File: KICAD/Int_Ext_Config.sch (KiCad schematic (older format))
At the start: 7 parts

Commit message: a ton of new stuff. V0.8
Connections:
- net labels added: +6V, +7V
- net labels removed: +2V5, VCC
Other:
- note added: "A voir au dernier moment"
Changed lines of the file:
@@
 $Descr A4 11693 8268
 encoding utf-8
-Sheet 8 15
+Sheet 8 16
 Title ""
 Date ""
@@
 Wire Wire Line
 	5450 3950 5450 4050
-$Comp
-L power:VCC #PWR0110
-U 1 1 618860AB
-P 5450 3950
-F 0 "#PWR0110" H 5450 3800 50  0001 C CNN
-F 1 "VCC" H 5465 4123 50  0000 C CNN
-F 2 "" H 5450 3950 50  0001 C CNN
-F 3 "" H 5450 3950 50  0001 C CNN
-	1    5450 3950
-	1    0    0    -1
-$EndComp
-$Comp
-L power:+2V5 #PWR0111
-U 1 1 618860B1
-P 5650 3950
-F 0 "#PWR0111" H 5650 3800 50  0001 C CNN
-F 1 "+2V5" H 5665 4123 50  0000 C CNN
-F 2 "" H 5650 3950 50  0001 C CNN
-F 3 "" H 5650 3950 50  0001 C CNN
-	1    5650 3950
-	1    0    0    -1
-$EndComp
 Text GLabel 5300 5150 2    50   Output ~ 0
 Ex_Rearm
@@
 Text GLabel 6100 2400 2    50   Output ~ 0
 CC_CV_Mode
-$Comp
-L power:VCC #PWR0112
-U 1 1 618860EA
-P 5600 1800
-F 0 "#PWR0112" H 5600 1650 50  0001 C CNN
-F 1 "VCC" H 5615 1973 50  0000 C CNN
-F 2 "" H 5600 1800 50  0001 C CNN
-F 3 "" H 5600 1800 50  0001 C CNN
-	1    5600 1800
-	1    0    0    -1
-$EndComp
 Wire Wire Line
 	5350 2400 5300 2400
@@
 Wire Wire Line
 	5000 4050 5450 4050
+Text Notes 4550 950  0    100  ~ 20
+A voir au dernier moment
+$Comp
+L Sesame:+7V #PWR0128
+U 1 1 61485513
+P 5600 1800
+F 0 "#PWR0128" H 5600 1650 50  0001 C CNN
+F 1 "+7V" H 5615 1973 50  0000 C CNN
+F 2 "" H 5600 1800 50  0001 C CNN
+F 3 "" H 5600 1800 50  0001 C CNN
+	1    5600 1800
+	1    0    0    -1
+$EndComp
+$Comp
+L Sesame:+7V #PWR0129
+U 1 1 61487244
+P 5450 3950
+F 0 "#PWR0129" H 5450 3800 50  0001 C CNN
+F 1 "+7V" H 5465 4123 50  0000 C CNN
+F 2 "" H 5450 3950 50  0001 C CNN
+F 3 "" H 5450 3950 50  0001 C CNN
+	1    5450 3950
+	1    0    0    -1
+$EndComp
+$Comp
+L power:+6V #PWR0130
+U 1 1 61487948
+P 5650 3950
+F 0 "#PWR0130" H 5650 3800 50  0001 C CNN
+F 1 "+6V" H 5665 4123 50  0000 C CNN
+F 2 "" H 5650 3950 50  0001 C CNN
+F 3 "" H 5650 3950 50  0001 C CNN
+	1    5650 3950
+	1    0    0    -1
+$EndComp
 $EndSCHEMATC

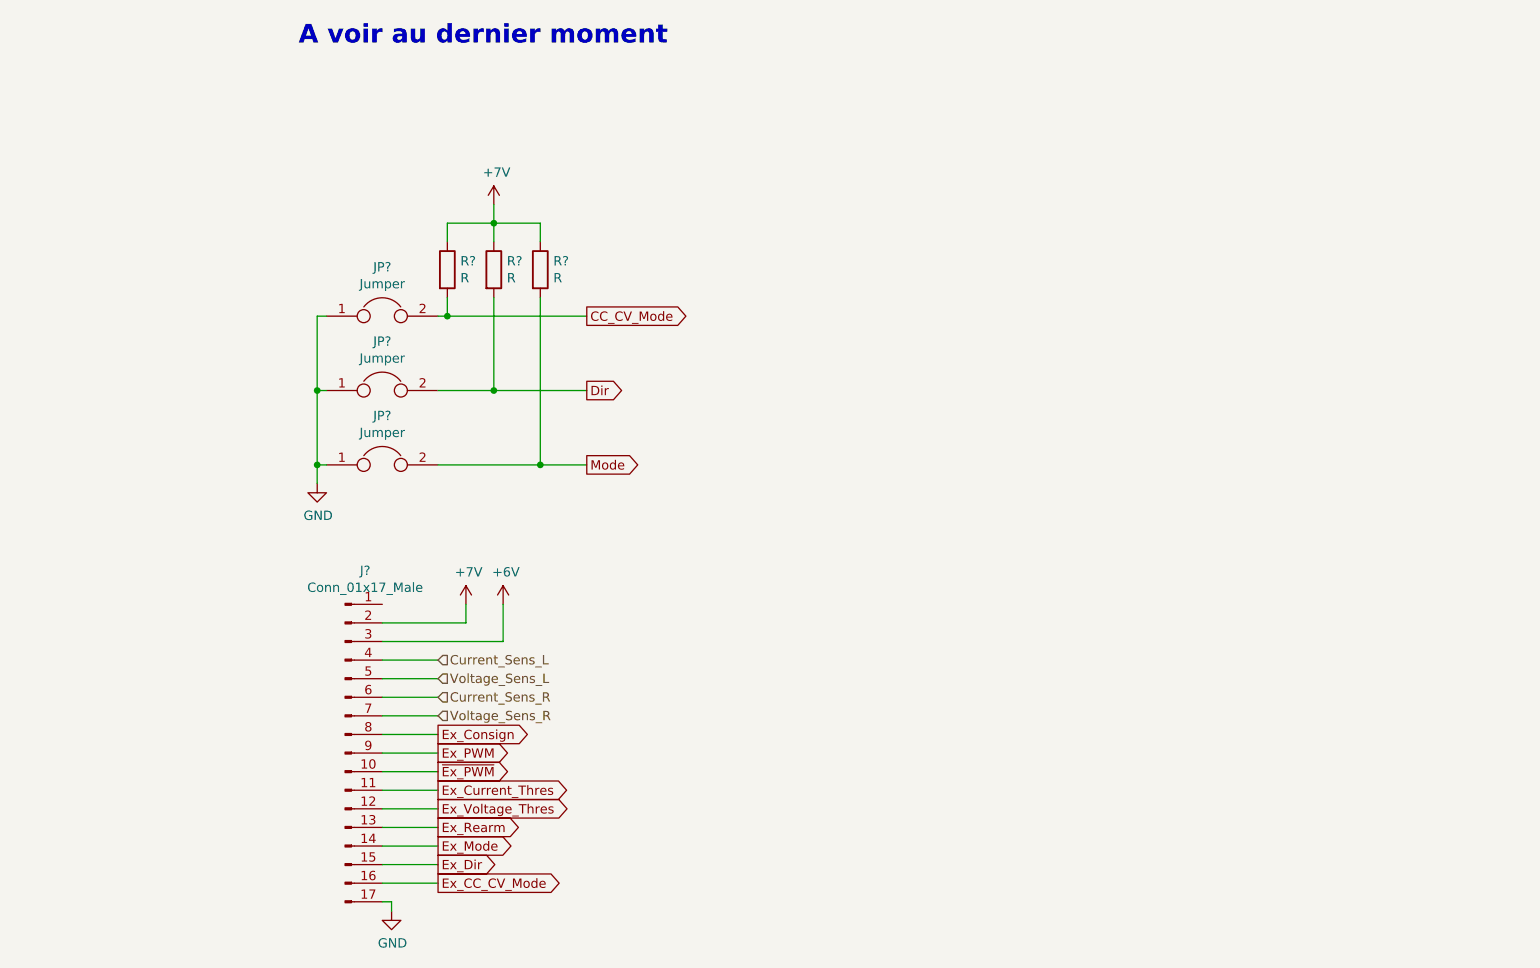
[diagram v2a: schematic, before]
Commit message: minor cleanup
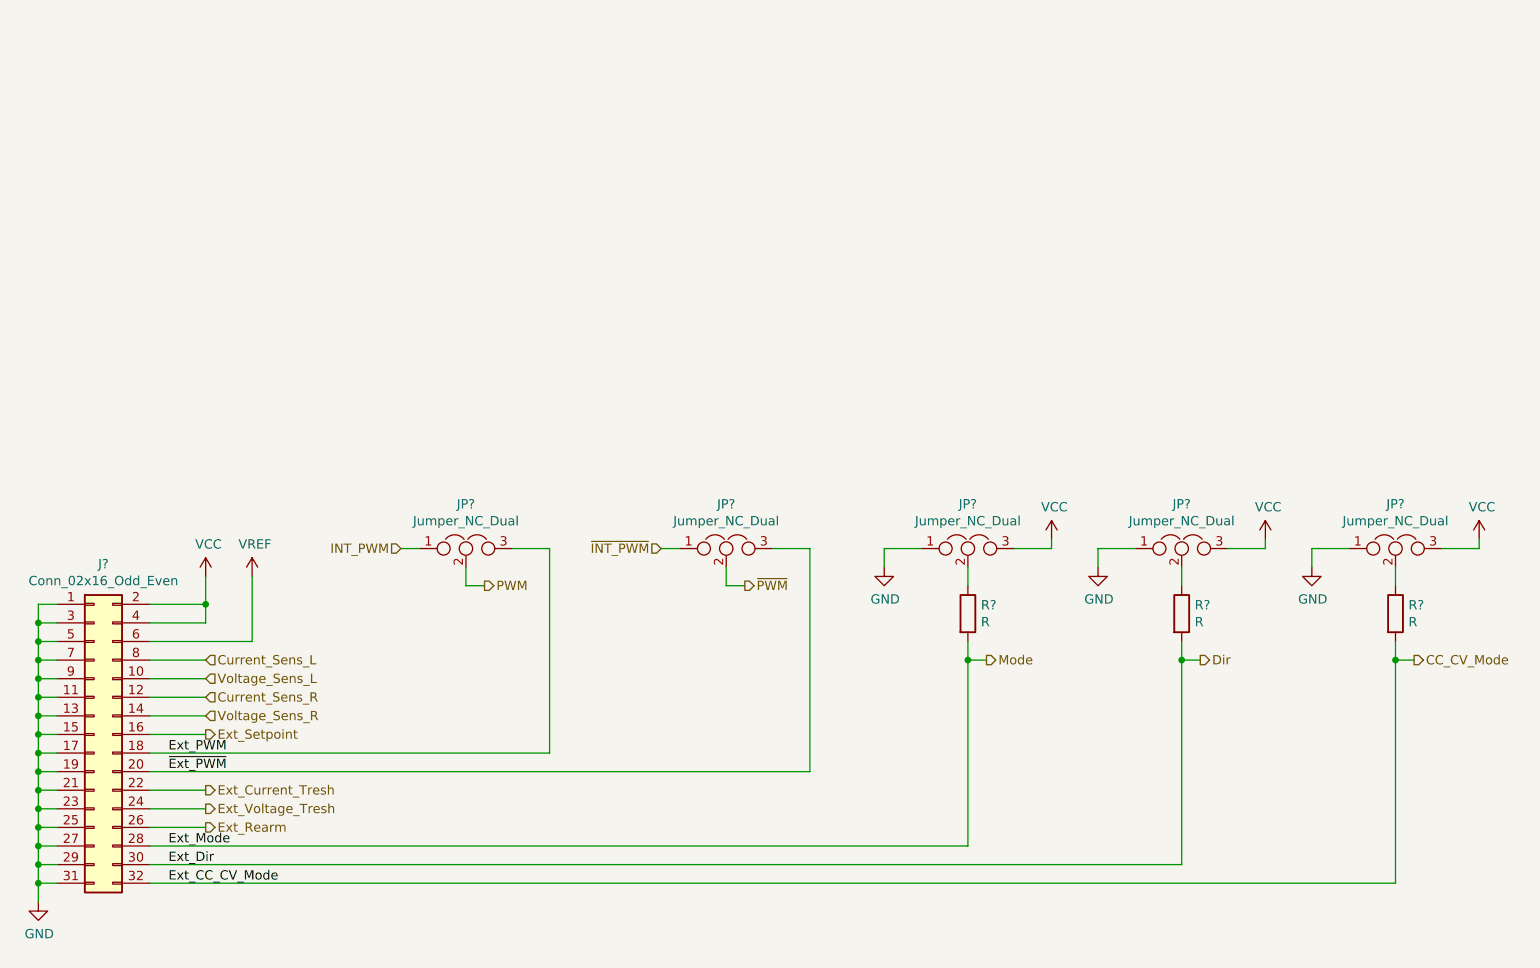
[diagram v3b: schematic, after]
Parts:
- removed J?: Conn_01x17_Male, symbol Connector:Conn_01x17_Male
- removed JP? (x3): Jumper, symbol Device:Jumper
- removed R? (x3): R, symbol Device:R
- added J?: Conn_02x16_Odd_Even, symbol Connector_Generic:Conn_02x16_Odd_Even
- added JP? (x5): Jumper_NC_Dual, symbol Device:Jumper_NC_Dual
- added R? (x3): R, symbol Device:R
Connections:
- net CC_CV_Mode: now also J?.32 (Pin_32), R?.2
- net Current_Sens_L: now also J?.8 (Pin_8)
- net Current_Sens_R: now also J?.12 (Pin_12)
- net Dir: now also J?.30 (Pin_30), R?.2
- net GND: now also J?.1 (Pin_1), J?.11 (Pin_11), J?.13 (Pin_13), J?.15 (Pin_15), J?.17 (Pin_17), J?.19 (Pin_19), J?.21 (Pin_21), J?.23 (Pin_23), J?.25 (Pin_25), J?.27 (Pin_27), J?.29 (Pin_29), J?.3 (Pin_3), J?.31 (Pin_31), J?.5 (Pin_5), J?.7 (Pin_7), J?.9 (Pin_9), JP?.1, JP?.1, JP?.1
- net Mode: now also J?.28 (Pin_28), R?.2
- net Voltage_Sens_L: now also J?.10 (Pin_10)
- net Voltage_Sens_R: now also J?.14 (Pin_14)
- new net: JP?.2, R?.1 (x3)
- new net Ext_Current_Tresh: J?.22 (Pin_22)
- new net Ext_PWM: J?.18 (Pin_18), JP?.3
- new net Ext_Rearm: J?.26 (Pin_26)
- new net Ext_Setpoint: J?.16 (Pin_16)
- new net Ext_Voltage_Tresh: J?.24 (Pin_24)
- new net INT_PWM: JP?.1
- new net PWM: JP?.2
- new net VCC: J?.2 (Pin_2), J?.4 (Pin_4), JP?.3, JP?.3, JP?.3
- new net VREF: J?.6 (Pin_6)
- new net ~Ext_PWM: J?.20 (Pin_20), JP?.3
- new net ~INT_PWM: JP?.1
- new net ~PWM: JP?.2
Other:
- note removed: "A voir au dernier moment"
